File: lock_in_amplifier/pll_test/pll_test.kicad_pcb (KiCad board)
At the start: 2 copper layers, 71.9 x 17.5 mm, 82 parts, among them J1 Conn_01x02, J2 Conn_01x04, J3 Conn_01x02, J36 DELAY SEL FINE, J37 DELAY SEL COARSE, U10 74HC4046A, U14 MCP6566, U15 MC74LCX16374, U5 74HC4040, U7 LM833

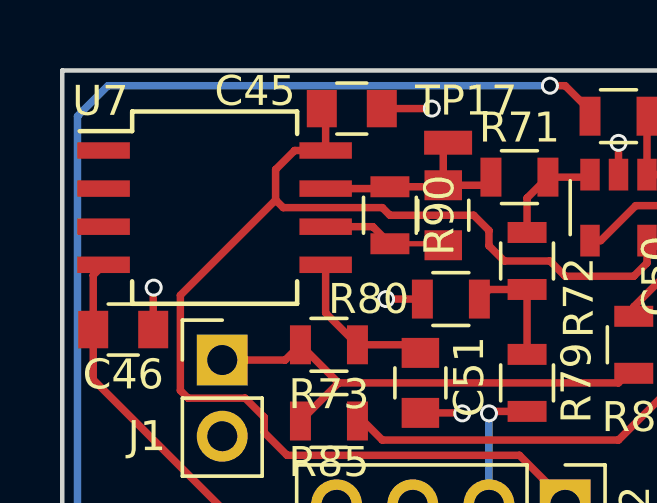
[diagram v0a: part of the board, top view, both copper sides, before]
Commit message: misc debug
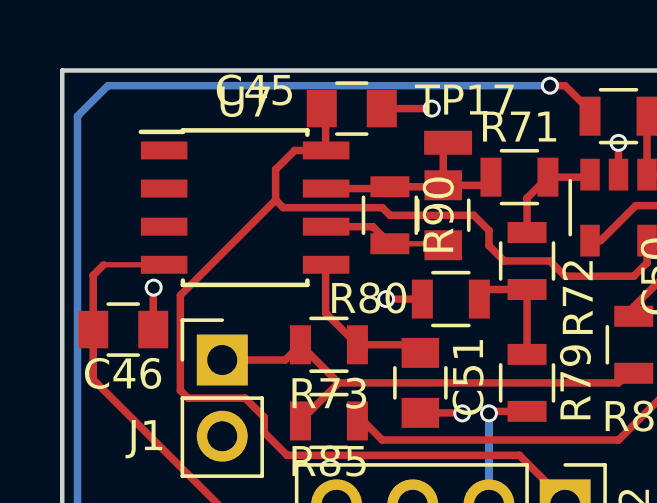
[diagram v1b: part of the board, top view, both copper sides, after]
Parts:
- U7: footprint Housings_SOIC:SO-8_5.3x6.2mm_Pitch1.27mm -> Housings_SOIC:SOIC-8_3.9x4.9mm_Pitch1.27mm
- moved U7 1.02 mm to (174.8, 94.2)
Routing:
- net /PLL/-5V: track 18.7 -> 21.2 mm
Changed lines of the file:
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@@
     (thickness 1.6)
     (drawings 10)
-    (tracks 542)
+    (tracks 544)
     (zones 0)
     (modules 82)
@@
     (34 B.Paste user)
     (35 F.Paste user)
-    (36 B.SilkS user)
+    (36 B.SilkS user hide)
     (37 F.SilkS user)
     (38 B.Mask user)
@@
     )
   )
-  (module Housings_SOIC:SO-8_5.3x6.2mm_Pitch1.27mm placed (layer F.Cu)
-    (at 173.736 94.234)
-    (descr "8-Lead Plastic Small Outline, 5.3x6.2mm Body (http://www.ti.com.cn/cn/lit/ds/symlink/tl7705a.pdf)")
-    (tags "SOIC 1.27")
-    (attr smd)
-    (fp_text reference U7 (at -3.81 -3.556) (layer F.SilkS)
-      (effects (font (size 1 1) (thickness 0.15)))
-    )
-    (fp_text value LM833 (at 0 4.13) (layer F.Fab)
-      (effects (font (size 1 1) (thickness 0.15)))
-    )
-    (fp_text user %R (at 0 0) (layer F.Fab)
-      (effects (font (size 1 1) (thickness 0.15)))
-    )
-    (fp_line (start -1.65 -3.1) (end 2.65 -3.1) (layer F.Fab) (width 0.15))
-    (fp_line (start 2.65 -3.1) (end 2.65 3.1) (layer F.Fab) (width 0.15))
-    (fp_line (start 2.65 3.1) (end -2.65 3.1) (layer F.Fab) (width 0.15))
-    (fp_line (start -2.65 3.1) (end -2.65 -2.1) (layer F.Fab) (width 0.15))
-    (fp_line (start -2.65 -2.1) (end -1.65 -3.1) (layer F.Fab) (width 0.15))
-    (fp_line (start -4.83 -3.35) (end -4.83 3.35) (layer F.CrtYd) (width 0.05))
-    (fp_line (start 4.83 -3.35) (end 4.83 3.35) (layer F.CrtYd) (width 0.05))
-    (fp_line (start -4.83 -3.35) (end 4.83 -3.35) (layer F.CrtYd) (width 0.05))
-    (fp_line (start -4.83 3.35) (end 4.83 3.35) (layer F.CrtYd) (width 0.05))
-    (fp_line (start -2.75 -3.205) (end -2.75 -2.55) (layer F.SilkS) (width 0.15))
-    (fp_line (start 2.75 -3.205) (end 2.75 -2.455) (layer F.SilkS) (width 0.15))
-    (fp_line (start 2.75 3.205) (end 2.75 2.455) (layer F.SilkS) (width 0.15))
-    (fp_line (start -2.75 3.205) (end -2.75 2.455) (layer F.SilkS) (width 0.15))
-    (fp_line (start -2.75 -3.205) (end 2.75 -3.205) (layer F.SilkS) (width 0.15))
-    (fp_line (start -2.75 3.205) (end 2.75 3.205) (layer F.SilkS) (width 0.15))
-    (fp_line (start -2.75 -2.55) (end -4.5 -2.55) (layer F.SilkS) (width 0.15))
-    (pad 1 smd rect (at -3.7 -1.905) (size 1.75 0.55) (layers F.Cu F.Paste F.Mask))
-    (pad 2 smd rect (at -3.7 -0.635) (size 1.75 0.55) (layers F.Cu F.Paste F.Mask))
-    (pad 3 smd rect (at -3.7 0.635) (size 1.75 0.55) (layers F.Cu F.Paste F.Mask))
-    (pad 4 smd rect (at -3.7 1.905) (size 1.75 0.55) (layers F.Cu F.Paste F.Mask)
-      (net 3 /PLL/-5V))
-    (pad 5 smd rect (at 3.7 1.905) (size 1.75 0.55) (layers F.Cu F.Paste F.Mask)
-      (net 8 "Net-(C51-Pad2)"))
-    (pad 6 smd rect (at 3.7 0.635) (size 1.75 0.55) (layers F.Cu F.Paste F.Mask)
-      (net 10 "Net-(C52-Pad2)"))
-    (pad 7 smd rect (at 3.7 -0.635) (size 1.75 0.55) (layers F.Cu F.Paste F.Mask)
-      (net 9 "Net-(C52-Pad1)"))
-    (pad 8 smd rect (at 3.7 -1.905) (size 1.75 0.55) (layers F.Cu F.Paste F.Mask)
-      (net 2 /PLL/+5V))
-    (model ${KISYS3DMOD}/Housings_SOIC.3dshapes/SO-8_5.3x6.2mm_Pitch1.27mm.wrl
-      (at (xyz 0 0 0))
-      (scale (xyz 1 1 1))
-      (rotate (xyz 0 0 0))
-    )
-  )
   (module Housings_SOIC:SOIC-16_3.9x9.9mm_Pitch1.27mm placed (layer F.Cu)
     (at 197.485 96.393 270)
@@
       (xy -0.113933 2.757629) (xy -0.013056 2.757714) (xy 0 2.757714) (xy 0.10391 2.757652)) (layer B.SilkS) (width 0.01))
   )
+  (module Housings_SOIC:SOIC-8_3.9x4.9mm_Pitch1.27mm (layer F.Cu)
+    (at 174.752 94.234)
+    (descr "8-Lead Plastic Small Outline (SN) - Narrow, 3.90 mm Body [SOIC] (see Microchip Packaging Specification 00000049BS.pdf)")
+    (tags "SOIC 1.27")
+    (attr smd)
+    (fp_text reference U7 (at 0 -3.5) (layer F.SilkS)
+      (effects (font (size 1 1) (thickness 0.15)))
+    )
+    (fp_text value LM833 (at 0 3.5) (layer F.Fab)
+      (effects (font (size 1 1) (thickness 0.15)))
+    )
+    (fp_text user %R (at 0 0) (layer F.Fab)
+      (effects (font (size 1 1) (thickness 0.15)))
+    )
+    (fp_line (start -0.95 -2.45) (end 1.95 -2.45) (layer F.Fab) (width 0.1))
+    (fp_line (start 1.95 -2.45) (end 1.95 2.45) (layer F.Fab) (width 0.1))
+    (fp_line (start 1.95 2.45) (end -1.95 2.45) (layer F.Fab) (width 0.1))
+    (fp_line (start -1.95 2.45) (end -1.95 -1.45) (layer F.Fab) (width 0.1))
+    (fp_line (start -1.95 -1.45) (end -0.95 -2.45) (layer F.Fab) (width 0.1))
+    (fp_line (start -3.73 -2.7) (end -3.73 2.7) (layer F.CrtYd) (width 0.05))
+    (fp_line (start 3.73 -2.7) (end 3.73 2.7) (layer F.CrtYd) (width 0.05))
+    (fp_line (start -3.73 -2.7) (end 3.73 -2.7) (layer F.CrtYd) (width 0.05))
+    (fp_line (start -3.73 2.7) (end 3.73 2.7) (layer F.CrtYd) (width 0.05))
+    (fp_line (start -2.075 -2.575) (end -2.075 -2.525) (layer F.SilkS) (width 0.15))
+    (fp_line (start 2.075 -2.575) (end 2.075 -2.43) (layer F.SilkS) (width 0.15))
+    (fp_line (start 2.075 2.575) (end 2.075 2.43) (layer F.SilkS) (width 0.15))
+    (fp_line (start -2.075 2.575) (end -2.075 2.43) (layer F.SilkS) (width 0.15))
+    (fp_line (start -2.075 -2.575) (end 2.075 -2.575) (layer F.SilkS) (width 0.15))
+    (fp_line (start -2.075 2.575) (end 2.075 2.575) (layer F.SilkS) (width 0.15))
+    (fp_line (start -2.075 -2.525) (end -3.475 -2.525) (layer F.SilkS) (width 0.15))
+    (pad 1 smd rect (at -2.7 -1.905) (size 1.55 0.6) (layers F.Cu F.Paste F.Mask))
+    (pad 2 smd rect (at -2.7 -0.635) (size 1.55 0.6) (layers F.Cu F.Paste F.Mask))
+    (pad 3 smd rect (at -2.7 0.635) (size 1.55 0.6) (layers F.Cu F.Paste F.Mask))
+    (pad 4 smd rect (at -2.7 1.905) (size 1.55 0.6) (layers F.Cu F.Paste F.Mask)
+      (net 3 /PLL/-5V))
+    (pad 5 smd rect (at 2.7 1.905) (size 1.55 0.6) (layers F.Cu F.Paste F.Mask)
+      (net 8 "Net-(C51-Pad2)"))
+    (pad 6 smd rect (at 2.7 0.635) (size 1.55 0.6) (layers F.Cu F.Paste F.Mask)
+      (net 10 "Net-(C52-Pad2)"))
+    (pad 7 smd rect (at 2.7 -0.635) (size 1.55 0.6) (layers F.Cu F.Paste F.Mask)
+      (net 9 "Net-(C52-Pad1)"))
+    (pad 8 smd rect (at 2.7 -1.905) (size 1.55 0.6) (layers F.Cu F.Paste F.Mask)
+      (net 2 /PLL/+5V))
+    (model ${KISYS3DMOD}/Housings_SOIC.3dshapes/SOIC-8_3.9x4.9mm_Pitch1.27mm.wrl
+      (at (xyz 0 0 0))
+      (scale (xyz 1 1 1))
+      (rotate (xyz 0 0 0))
+    )
+  )
   (gr_text "BOARD VER. 1.0\nC1:___\nR1:___\nR2:___\nPH. CMP: 123" (at 189.611 96.0628) (layer B.SilkS)
     (effects (font (size 1.5 1.5) (thickness 0.3)) (justify left mirror))
@@
   (segment (start 177.436 92.329) (end 177.436 91.06) (width 0.25) (layer F.Cu) (net 2))
   (segment (start 177.436 91.06) (end 177.308 90.932) (width 0.25) (layer F.Cu) (net 2))
+  (segment (start 172.052 96.139) (end 170.036 96.139) (width 0.1778) (layer F.Cu) (net 3) (status 400000))
+  (segment (start 170.036 96.139) (end 169.688 96.487) (width 0.1778) (layer F.Cu) (net 3))
   (segment (start 169.688 98.298) (end 169.688 99.965) (width 0.25) (layer F.Cu) (net 3))
   (segment (start 180.34 105.41) (end 180.34 104.14) (width 0.25) (layer F.Cu) (net 3))
